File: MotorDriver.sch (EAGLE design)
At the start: 144 parts, among them IC3 STM32F071V8T6V8, J10 B4B-PH-K-S(LF)(SN), J11 B4B-PH-K-S(LF)(SN), J12 B4B-PH-K-S(LF)(SN), J13 B4B-PH-K-S(LF)(SN), J14 B4B-PH-K-S(LF)(SN), J15 B4B-PH-K-S(LF)(SN), J16 B4B-PH-K-S(LF)(SN), J18 B2P-VH(LF)(SN), J19 B2P-VH(LF)(SN), J20 B2P-VH(LF)(SN), J21 B2P-VH(LF)(SN), J22 B2P-VH(LF)(SN), J23 B2P-VH(LF)(SN), J24 B2P-VH(LF)(SN), J25 B2P-VH(LF)(SN), J26 XT30PWXT30PW, J9 B4B-PH-K-S(LF)(SN), M0 VNH7100ASTR, M1 VNH7100ASTR, M2 VNH7100ASTR, M3 VNH7100ASTR, M4 VNH7100ASTR, M5 VNH7100ASTR, M6 VNH7100ASTR, M7 VNH7100ASTR, Q2 20V/4.2A/52mΩ/1.4W, U1 ICE5LP1K-SG48ITR, U10 LD1085D2T33R, U11 LD1085D2T33R, U2 N25Q032A13ESC40F, U3 BD9D323QWZ-E2, U4 BD9D323QWZ-E2, U5 MMDT5401-7-F, U6 BD9D323QWZ-E2, U7 MIC5504-3.3YM5-TR, U8 MIC5365-1.2YC5-TR, U9 LD1085D2T33R, X1 MINI-USB-UX60-MB-5S8, Y1 ECS-TXO-2520-33-160-AN-TR, Y2 32.768kHz, Y4 CRYSTAL-GROUNDEDSMD-3.2X2.5

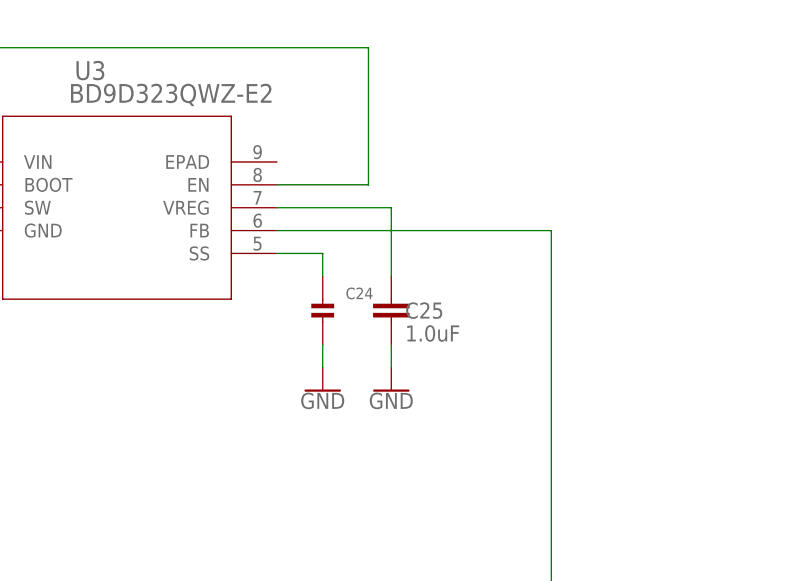
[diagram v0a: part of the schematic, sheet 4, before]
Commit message: update
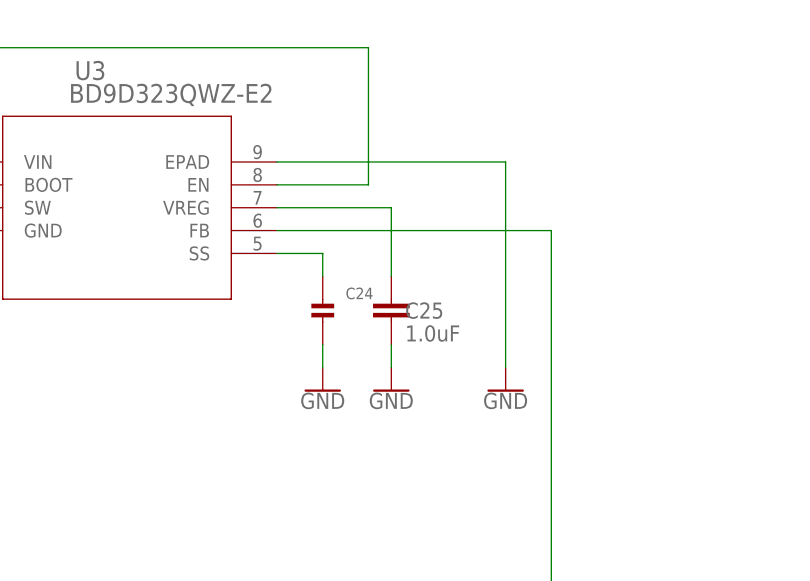
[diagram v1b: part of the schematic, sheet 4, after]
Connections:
- net GND: now also U3.EPAD, U6.EPAD
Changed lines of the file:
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@@
 <part name="C55" library="SparkFun-Capacitors" deviceset="22PF" device="-0603-50V-5%" value=""/>
 <part name="GND88" library="SparkFun-PowerSymbols" deviceset="GND" device=""/>
+<part name="GND89" library="SparkFun-PowerSymbols" deviceset="GND" device=""/>
+<part name="GND90" library="SparkFun-PowerSymbols" deviceset="GND" device=""/>
 </parts>
 <sheets>
@@
 <attribute name="VALUE" x="172.72" y="-66.294" size="1.778" layer="96" align="top-center"/>
 </instance>
+<instance part="GND89" gate="1" x="-2.54" y="53.34" smashed="yes">
+<attribute name="VALUE" x="-2.54" y="53.086" size="1.778" layer="96" align="top-center"/>
+</instance>
 </instances>
 <busses>
@@
 <wire x1="172.72" y1="-40.64" x2="172.72" y2="-63.5" width="0.1524" layer="91"/>
 </segment>
+<segment>
+<pinref part="U3" gate="A" pin="EPAD"/>
+<wire x1="-27.94" y1="78.74" x2="-2.54" y2="78.74" width="0.1524" layer="91"/>
+<wire x1="-2.54" y1="78.74" x2="-2.54" y2="55.88" width="0.1524" layer="91"/>
+<pinref part="GND89" gate="1" pin="GND"/>
+</segment>
 </net>
 <net name="N$20" class="0">
@@
 <attribute name="VALUE" x="160.02" y="45.974" size="1.778" layer="96" align="bottom-center"/>
 </instance>
+<instance part="GND90" gate="1" x="22.86" y="22.86" smashed="yes">
+<attribute name="VALUE" x="22.86" y="22.606" size="1.778" layer="96" align="top-center"/>
+</instance>
 </instances>
 <busses>
@@
 <wire x1="-83.82" y1="-63.5" x2="-83.82" y2="-86.36" width="0.1524" layer="91"/>
 </segment>
+<segment>
+<pinref part="U6" gate="A" pin="EPAD"/>
+<wire x1="0" y1="48.26" x2="22.86" y2="48.26" width="0.1524" layer="91"/>
+<wire x1="22.86" y1="48.26" x2="22.86" y2="25.4" width="0.1524" layer="91"/>
+<pinref part="GND90" gate="1" pin="GND"/>
+</segment>
 </net>
